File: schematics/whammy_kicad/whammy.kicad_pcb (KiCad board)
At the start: 2 copper layers, 120 x 100 mm, 60 parts, among them J2 Conn_01x03, J3 Conn_01x03, J5 Conn_01x03, Q1 2SK2013, Q2 2SJ313, Q3 2SK2013, Q4 2SJ313, U1 OPA2604, U4 4N35, U5 4N35

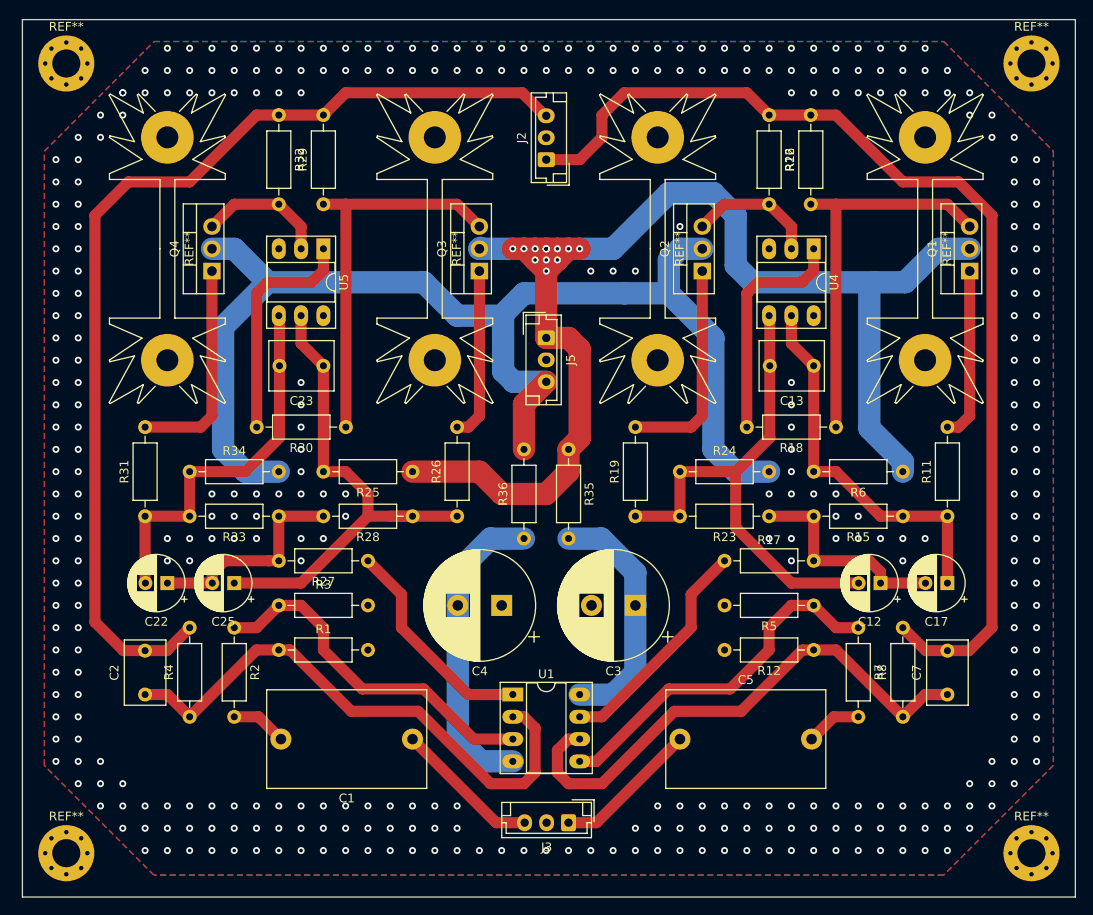
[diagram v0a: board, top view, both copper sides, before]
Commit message: Final version
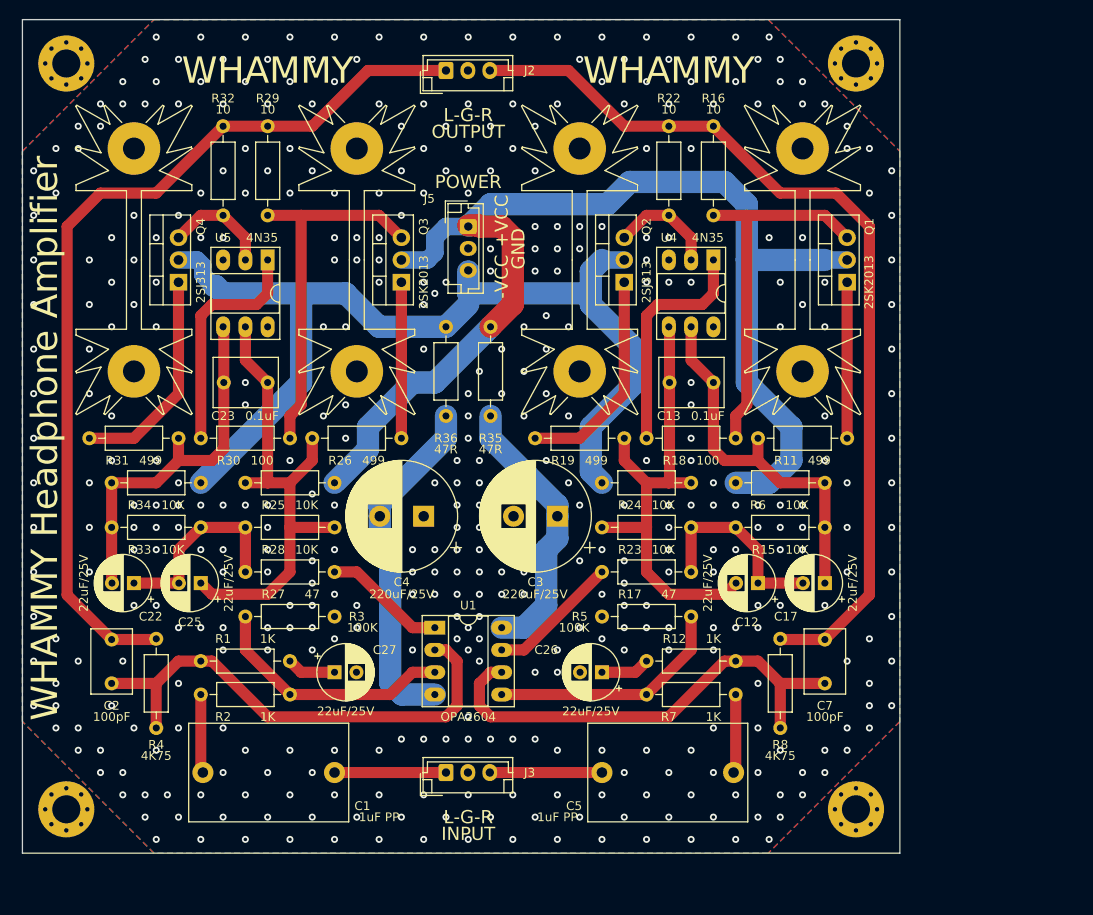
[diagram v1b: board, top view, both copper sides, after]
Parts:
- removed the REF** at (195.0, 140.0)
- removed the REF** at (195.0, 50.0)
- added ?: MountingHole_3.2mm_M3_Pad_Via, MountingHole:MountingHole_3.2mm_M3_Pad_Via, F.Cu at (175.0, 135.0)
- added ?: MountingHole_3.2mm_M3_Pad_Via, MountingHole:MountingHole_3.2mm_M3_Pad_Via, F.Cu at (175.0, 50.0)
- added C26: 22uF/25V, Capacitor_THT:CP_Radial_D6.3mm_P2.50mm, F.Cu at (146.1, 119.4)
- added C27: 22uF/25V, Capacitor_THT:CP_Radial_D6.3mm_P2.50mm, F.Cu at (115.6, 119.4)
- C3, C4: value 220uF/50V -> 220uF/25V
- moved R7 25.3 mm to (151.1, 121.9), turned to 0 degrees
- moved R11 23.3 mm to (163.8, 92.7), turned to 0 degrees
- moved R6 19.1 mm to (161.3, 97.8), turned to 0 degrees
- moved R26 18.8 mm to (113.0, 92.7), turned to 0 degrees
- moved R35 16.6 mm to (133.3, 80.0)
- moved R36 16.6 mm to (128.3, 90.2)
- moved J5 15.5 mm to (130.8, 68.6)
- moved J2 15.3 mm to (128.3, 50.8), turned to 0 degrees
- moved J3 15.1 mm to (128.3, 130.8), turned to 0 degrees
- moved C7 14.0 mm to (171.4, 120.7)
- moved Q1 14.0 mm to (174.0, 74.9)
- moved R17 14.0 mm to (146.1, 108.0)
- moved R5 14.0 mm to (156.2, 113.0)
- moved R8 14.0 mm to (166.4, 125.7)
- moved REF** 14.0 mm to (168.9, 72.4)
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- renumbered REF** to ?
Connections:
- J2 pad 1: LEFT_OUT -> RIGHT_OUT
- J2 pad 3: RIGHT_OUT -> LEFT_OUT
- J3 pad 1: Net-(C5-Pad1) -> Net-(C1-Pad1)
- J3 pad 3: Net-(C1-Pad1) -> Net-(C5-Pad1)
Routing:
- net -15V: track 140.8 -> 113.8 mm
- net +15V: track 154.9 -> 138.7 mm, vias 13 -> 0
- net LEFT_OUT: track 120.6 -> 104.9 mm
- net Net-(R5-Pad1): track 41.7 -> 27.5 mm
- net RIGHT_OUT: track 117.9 -> 104.8 mm
- net Net-(R2-Pad1): track 40.6 -> 28.6 mm
- net Net-(R17-Pad1): track 26.1 -> 15.1 mm
- net Net-(R27-Pad1): track 25.1 -> 14.1 mm
- net Net-(C2-Pad1): track 63.6 -> 56.8 mm
- net Net-(C7-Pad1): track 61.1 -> 54.3 mm
- net Net-(C27-Pad1): track 0.00 -> 5.61 mm
- net Net-(C26-Pad1): track 0.00 -> 5.61 mm
- net Net-(C4-Pad2): track 35.5 -> 39.7 mm
- net Net-(C1-Pad1): track 16.7 -> 12.7 mm
- net Net-(C5-Pad1): track 16.6 -> 12.8 mm
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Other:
- board size 120 x 100 mm -> 100 x 95 mm
- net class Power added: clearance 0.5, trace_width 0.25, via_dia 0.8, via_drill 0.4
- board text added: "+VCC"
- board text added: "-VCC"
- board text added: "GND"
- board text added: "INPUT"
- board text added: "L-G-R"
- board text added: "OUTPUT"
- board text added: "POWER"
- board text added: "WHAMMY"
- board text added: "WHAMMY Headphone Amplifier"
